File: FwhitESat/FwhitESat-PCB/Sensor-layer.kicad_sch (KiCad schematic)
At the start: 4 parts, among them U2 BMP180, U3 DS1307_, U6 GPS-NEO6M, U7 MPU-6050

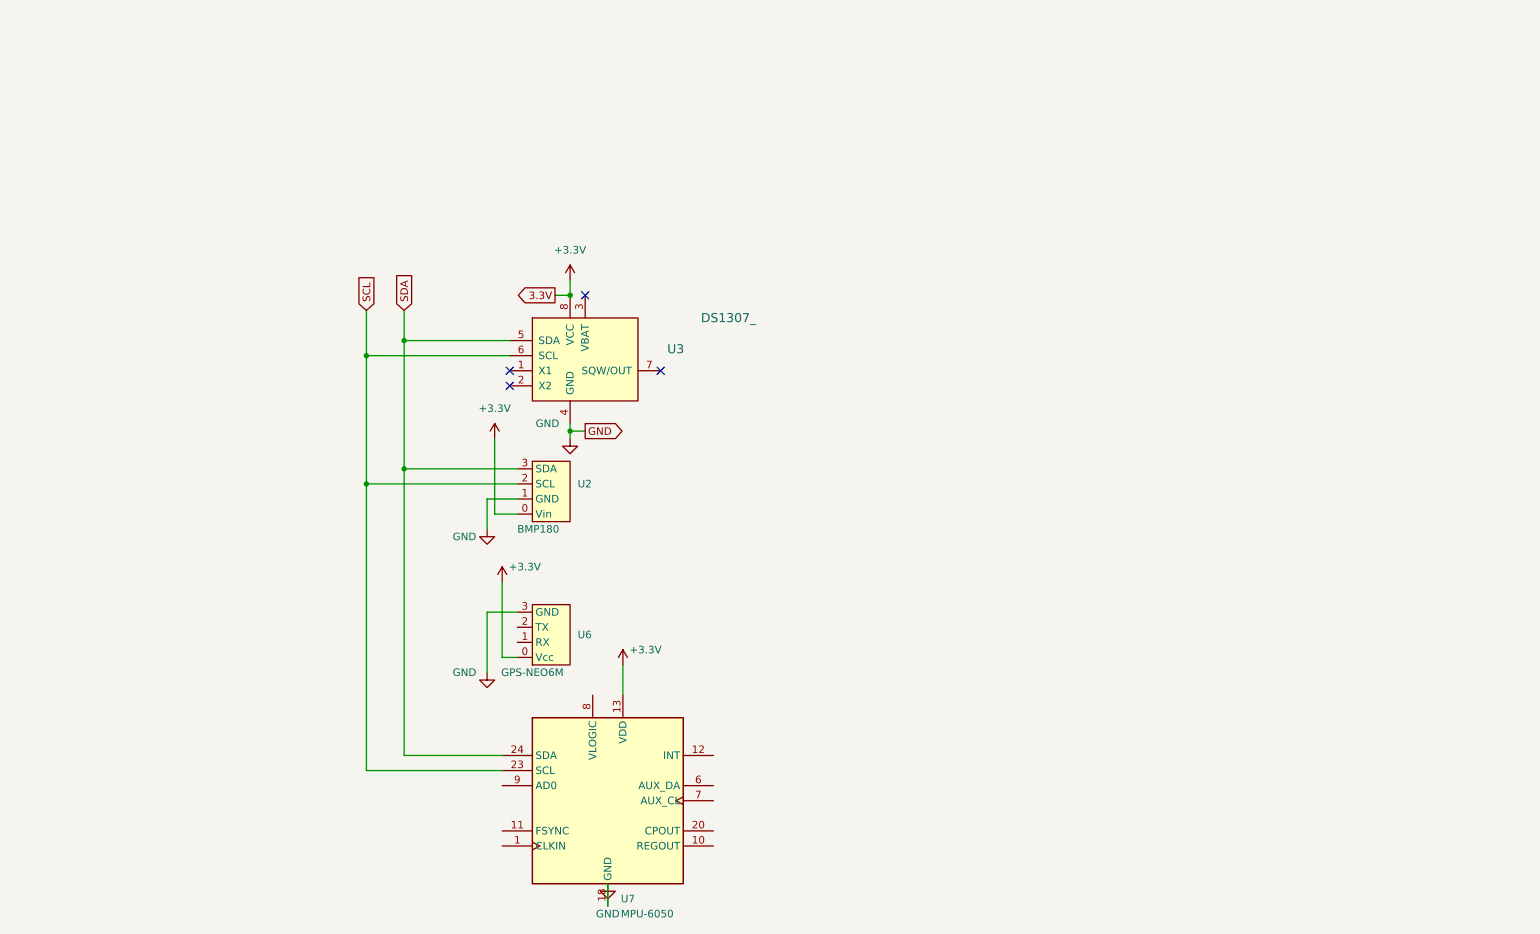
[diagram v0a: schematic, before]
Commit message: おなかすいた
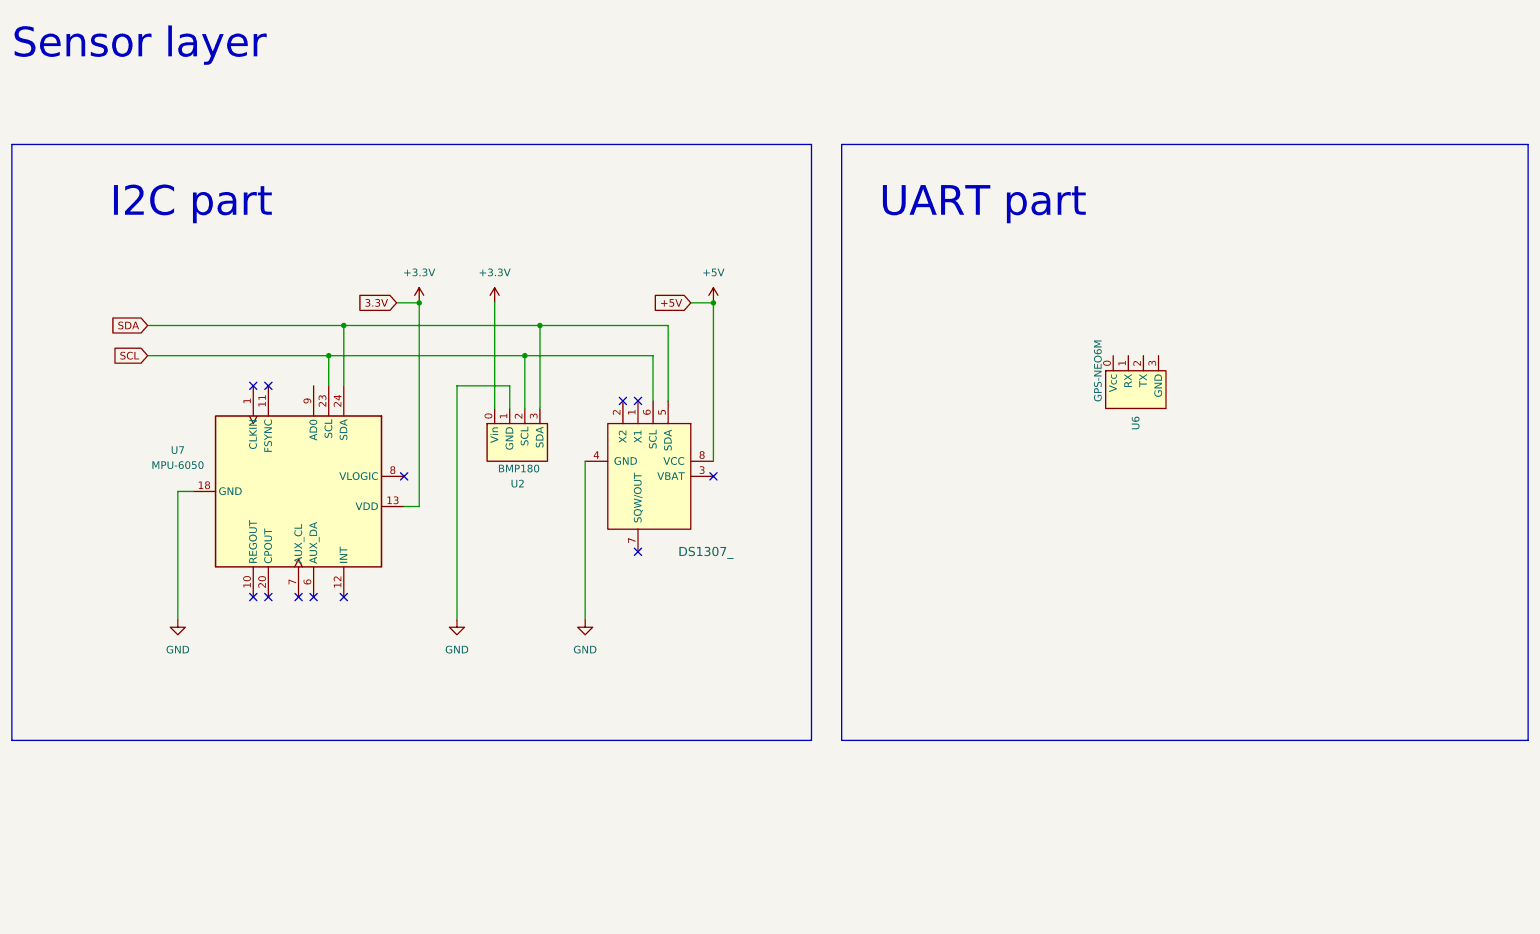
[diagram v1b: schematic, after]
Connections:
- net +3.3V: no longer U3.8 (VCC), U6.0 (Vcc)
- net GND: no longer U6.3 (GND)
- new net +5V: U3.8 (VCC)
- no-connect marks 4 -> 12
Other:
- note added: "I2C part"
- note added: "Sensor layer"
- note added: "UART part"
- moved on the sheet: U2, U6, U7
